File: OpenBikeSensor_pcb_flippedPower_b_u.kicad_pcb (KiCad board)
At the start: 2 copper layers, 62.8 x 62.2 mm, 35 parts, among them J1 Conn_01x02_Male, J10 Conn_02x03_Odd_Even, J11 Conn_01x02_Male, J2 Conn_01x04_Female, J3 Conn_01x04_Male, J4 Conn_01x04_Male, J5 Conn_01x05_Male, J6 Conn_01x02_Male, J7 Conn_01x06_Male, J8 Conn_01x06_Male, J9 Conn_01x06_Male, M1 LIPoChargerwithProtection, Q1 BS170, U1 ESP32-DEVKIT-32C, U3 XUNPU-TF-115-C266620, U4 DCDC_fix

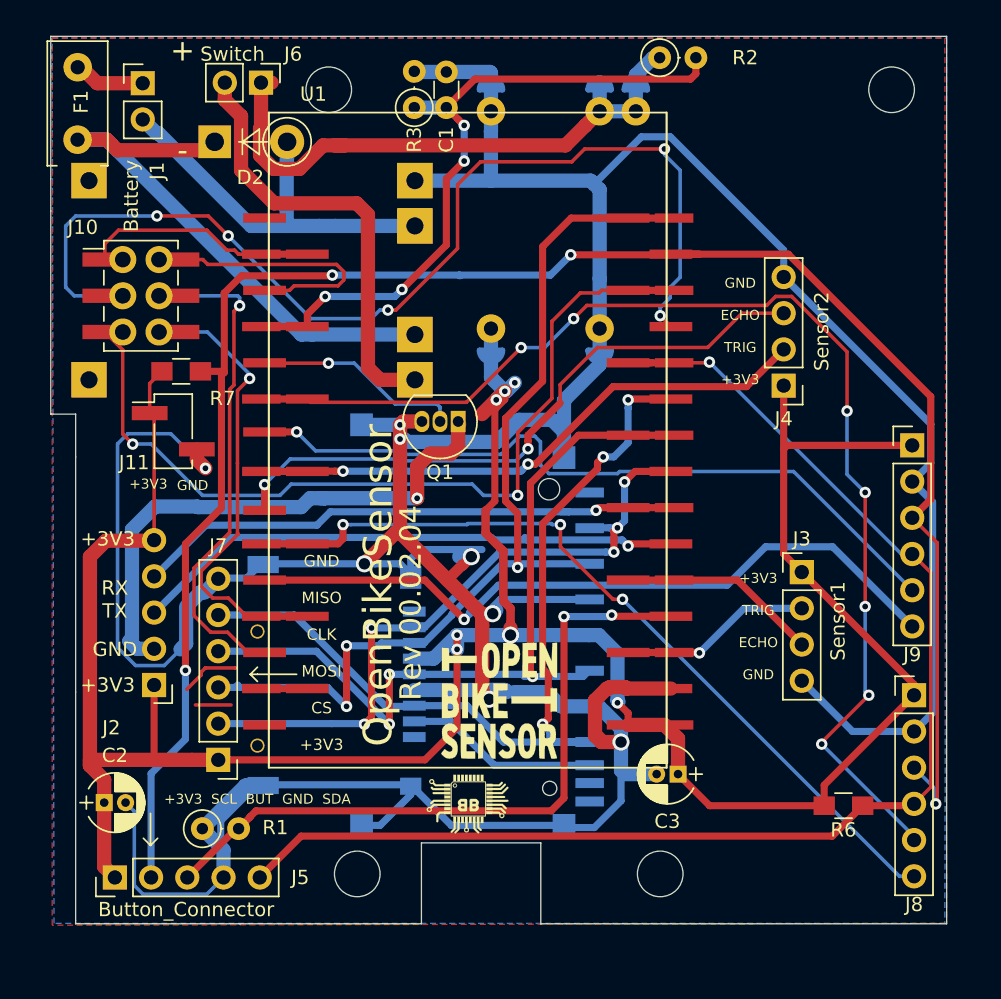
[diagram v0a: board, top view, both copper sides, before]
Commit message: new _u version
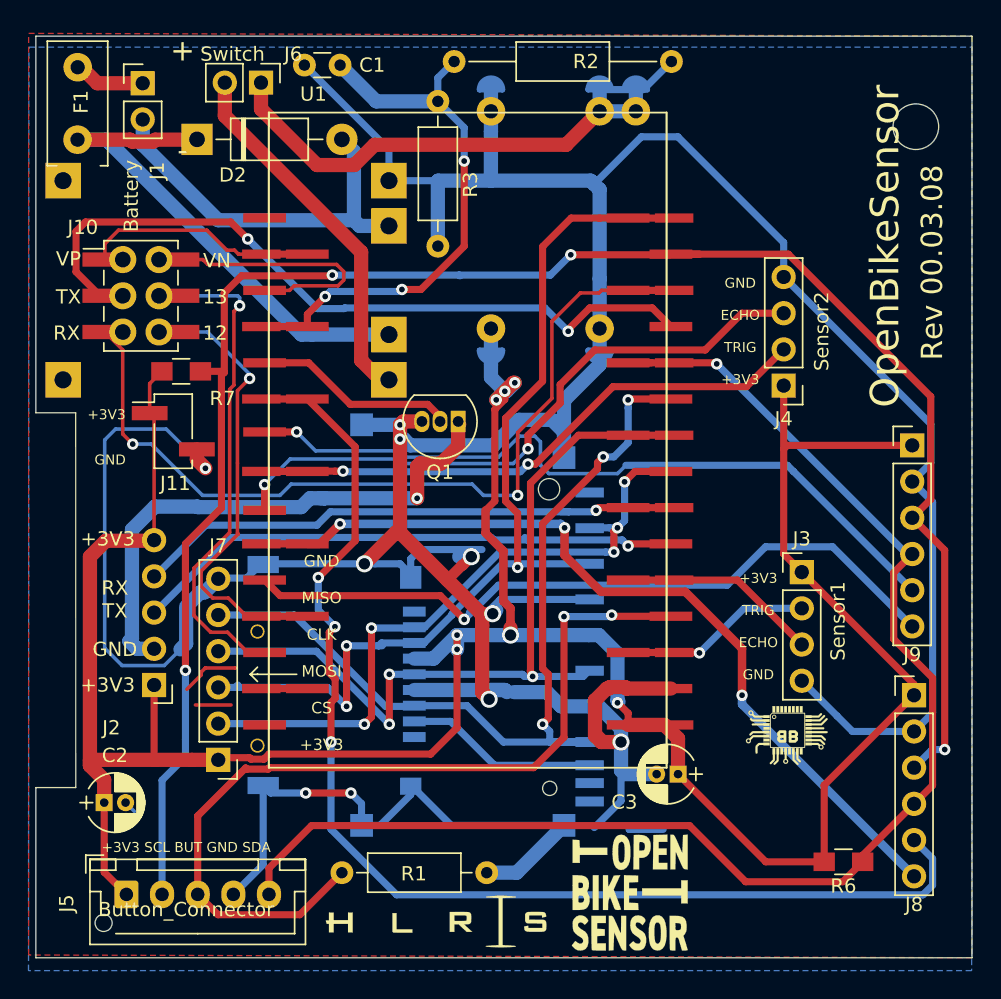
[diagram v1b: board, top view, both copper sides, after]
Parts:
- removed the REF** at (81.2, 50.7)
- removed the REF** at (41.8, 50.8)
- removed the REF** at (43.8, 105.8)
- added G***: LOGO, HLRS_LogoBack:HLRS_LogoBack, F.Cu at (80.3, 64.1)
- added G***: LOGO, HLRS_Logo:HLRS_Logo, F.Cu at (49.3, 109.1)
- D2: footprint Diodes_THT:D_DO-41_SOD81_P5.08mm_Vertical_KathodeUp -> Diode_THT:D_DO-41_SOD81_P10.16mm_Horizontal
- J5: footprint Pin_Headers:Pin_Header_Straight_1x05_Pitch2.54mm -> Connector_JST:JST_XH_B5B-XH-AM_1x05_P2.50mm_Vertical
- R1, R3: footprint Resistors_THT:R_Axial_DIN0207_L6.3mm_D2.5mm_P2.54mm_Vertical -> Resistor_THT:R_Axial_DIN0207_L6.3mm_D2.5mm_P10.16mm_Horizontal
- R2: footprint Resistors_THT:R_Axial_DIN0207_L6.3mm_D2.5mm_P2.54mm_Vertical -> Resistor_THT:R_Axial_DIN0207_L6.3mm_D2.5mm_P15.24mm_Horizontal
- moved REF** 55.4 mm to (82.9, 53.3)
- moved G*** 46.1 mm to (71.6, 55.4), turned to 270 degrees
- moved G*** 22.9 mm to (73.8, 95.9)
- moved G*** 20.7 mm to (72.0, 102.4), turned to 90 degrees
- moved R1 20.2 mm to (52.8, 105.7), turned to 180 degrees
- moved G*** 16.3 mm to (62.9, 107.1)
- moved C1 8.03 mm to (42.5, 49.0), turned to 180 degrees
- moved R6 3.94 mm to (77.9, 104.9)
- moved M1 1.82 mm to (35.2, 64.1)
- moved R3 1.71 mm to (49.4, 51.6), turned to 270 degrees
- moved J5 1.44 mm to (27.6, 107.2), turned to 0 degrees
- moved D2 1.25 mm to (32.5, 54.2)
- moved R2 0.87 mm to (65.8, 48.8), turned to 180 degrees
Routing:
- net TX: track 75.3 -> 52.2 mm, vias 5 -> 2
- net BUTTON: track 49.0 -> 61.5 mm
- net Net-(C1-Pad1): track 48.4 -> 39.2 mm, vias 4 -> 3
- net +3V3: track 223.8 -> 229.9 mm
- net SDA: track 93.7 -> 99.3 mm
- net Net-(J6-Pad2): track 31.2 -> 26.0 mm
- net +BATT: track 39.3 -> 35.8 mm
- net SCL: track 134.8 -> 131.5 mm
- net XSHUT_1: track 58.1 -> 60.0 mm
- net GND: track 337.7 -> 335.9 mm, vias 8 -> 10
- net -BATT: track 28.5 -> 27.4 mm
- net +VDC: track 41.2 -> 40.2 mm
- net GPIO_INT_2: track 52.2 -> 52.7 mm
- net GPS_GND_CONT: track 14.6 -> 14.2 mm, vias 1 -> 0
- net GPIO_INT_1: track 84.8 -> 85.1 mm, vias 7 -> 3
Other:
- board size 62.8 x 62.2 mm -> 65.7 x 64.6 mm
- board text added: "12"
- board text added: "13"
- board text added: "RX"
- board text added: "Rev 00.03.08"
- board text added: "TX"
- board text added: "VN"
- board text added: "VP"
- board text removed: "Rev 00.02.04"
